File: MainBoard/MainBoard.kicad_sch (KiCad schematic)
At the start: 43 parts, among them J1 1761681-3, Q1 BC557, U1 LM393, U2 TL074

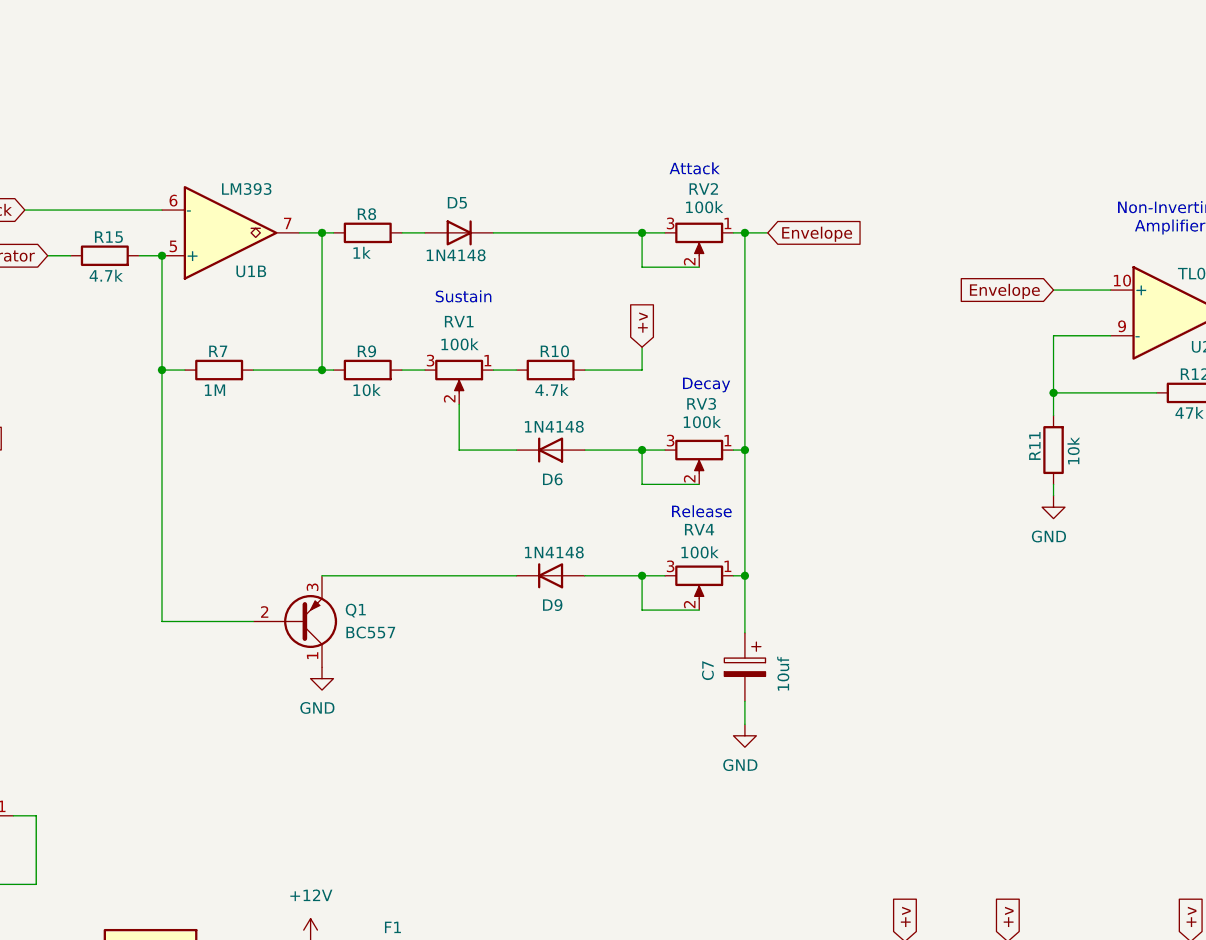
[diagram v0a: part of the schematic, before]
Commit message: testing
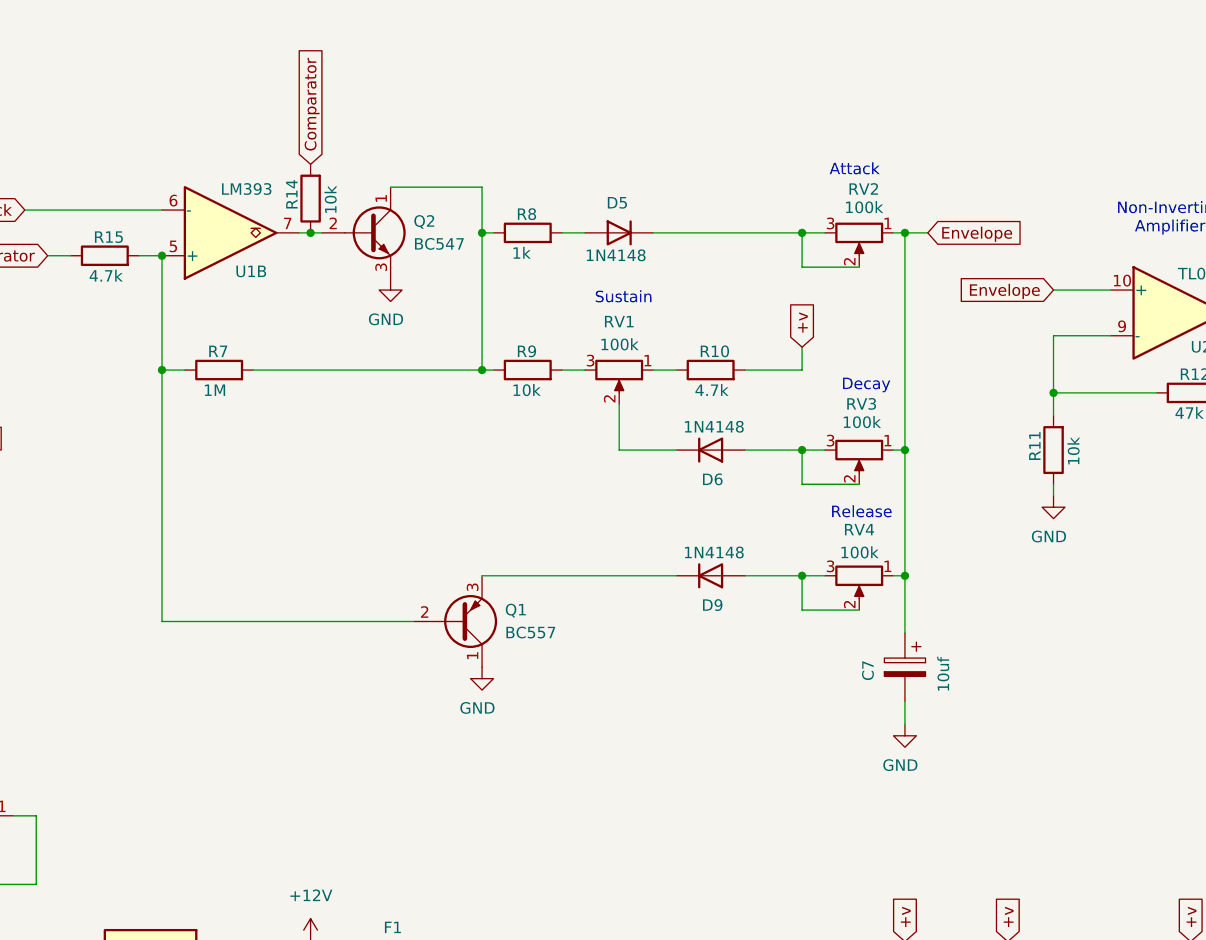
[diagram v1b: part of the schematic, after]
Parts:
- added Q2: BC547, Package_TO_SOT_THT:TO-92_Inline, symbol Transistor_BJT:BC547
- added R14: 10k, symbol Device:R
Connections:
- net Comparator: now also R14.2
- net GND: now also Q2.3 (E)
- net at R7.2, R8.1, R9.1: now also Q2.1 (C); no longer U1.7
- new net: Q2.2 (B), R14.1, U1.7
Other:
- moved on the sheet: C7, D5, D6, D9, Q1, R10, R8, R9, RV1, RV2, RV3, RV4
